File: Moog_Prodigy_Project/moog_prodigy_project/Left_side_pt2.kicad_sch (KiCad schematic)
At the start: 61 parts, among them Q1 CA3046, Q15 BC549, Q2 CA3046, Q4 CA3046, Q6 BC549, SW1 Switch_4x4, SW4 Switch_4x4, U2A1 OPA134, U2B3 OPA134, U5 NE5532, U6 LT1011CN8, U7 AD8066ARM, U8 NE5532

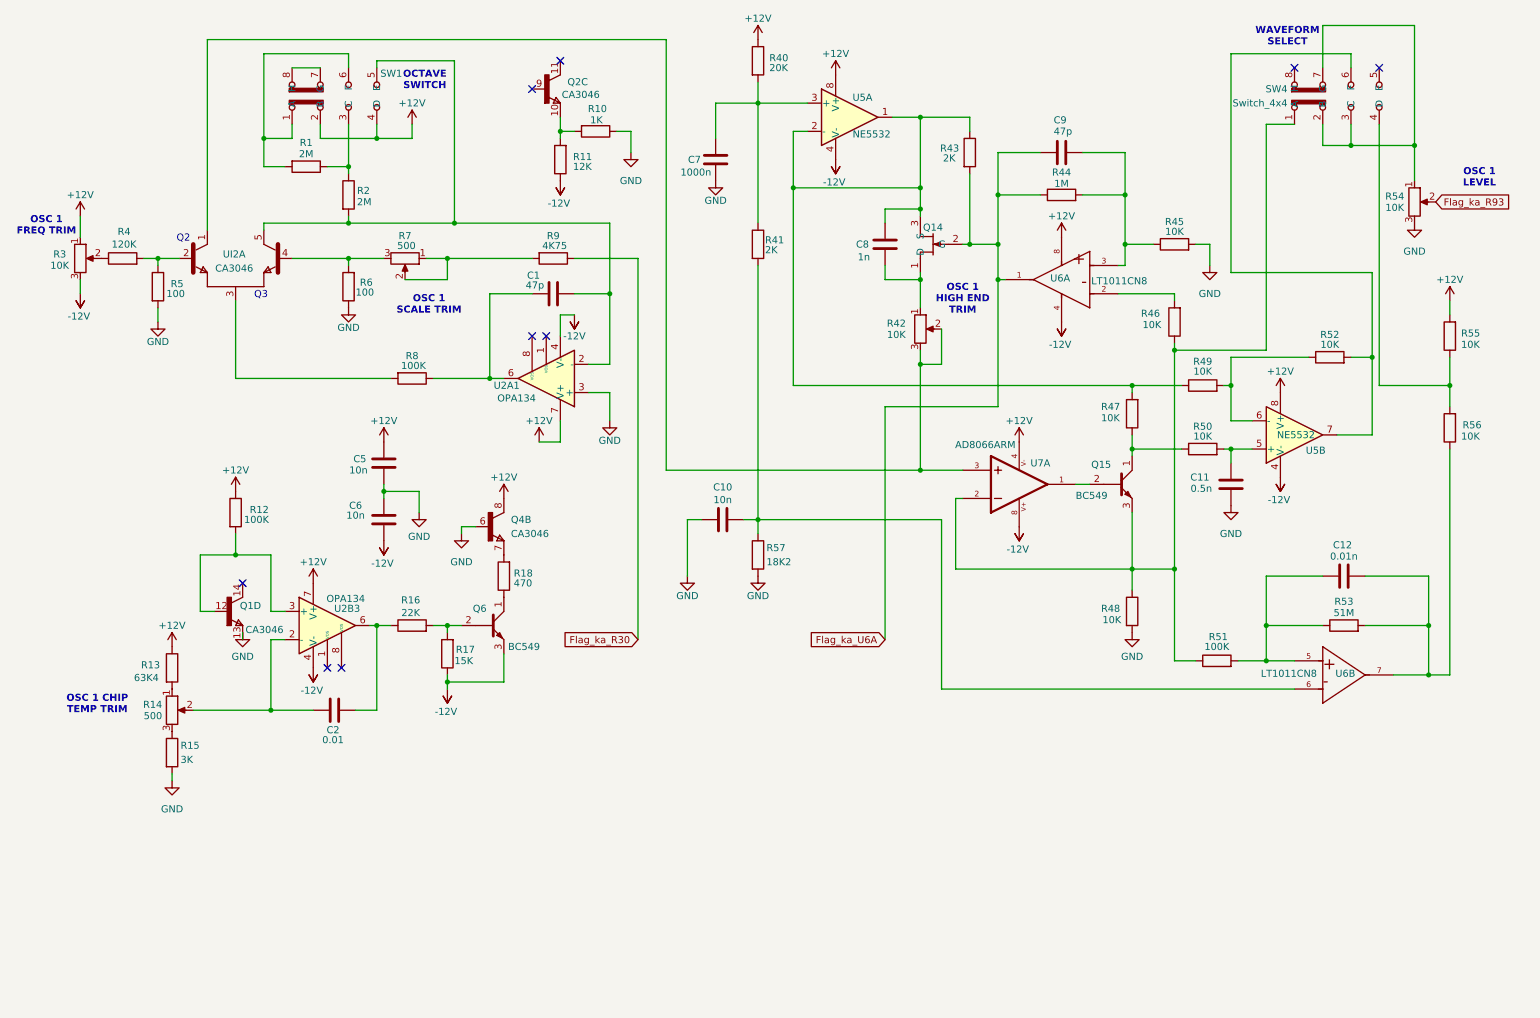
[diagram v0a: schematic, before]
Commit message: Spajanje projekta final 1
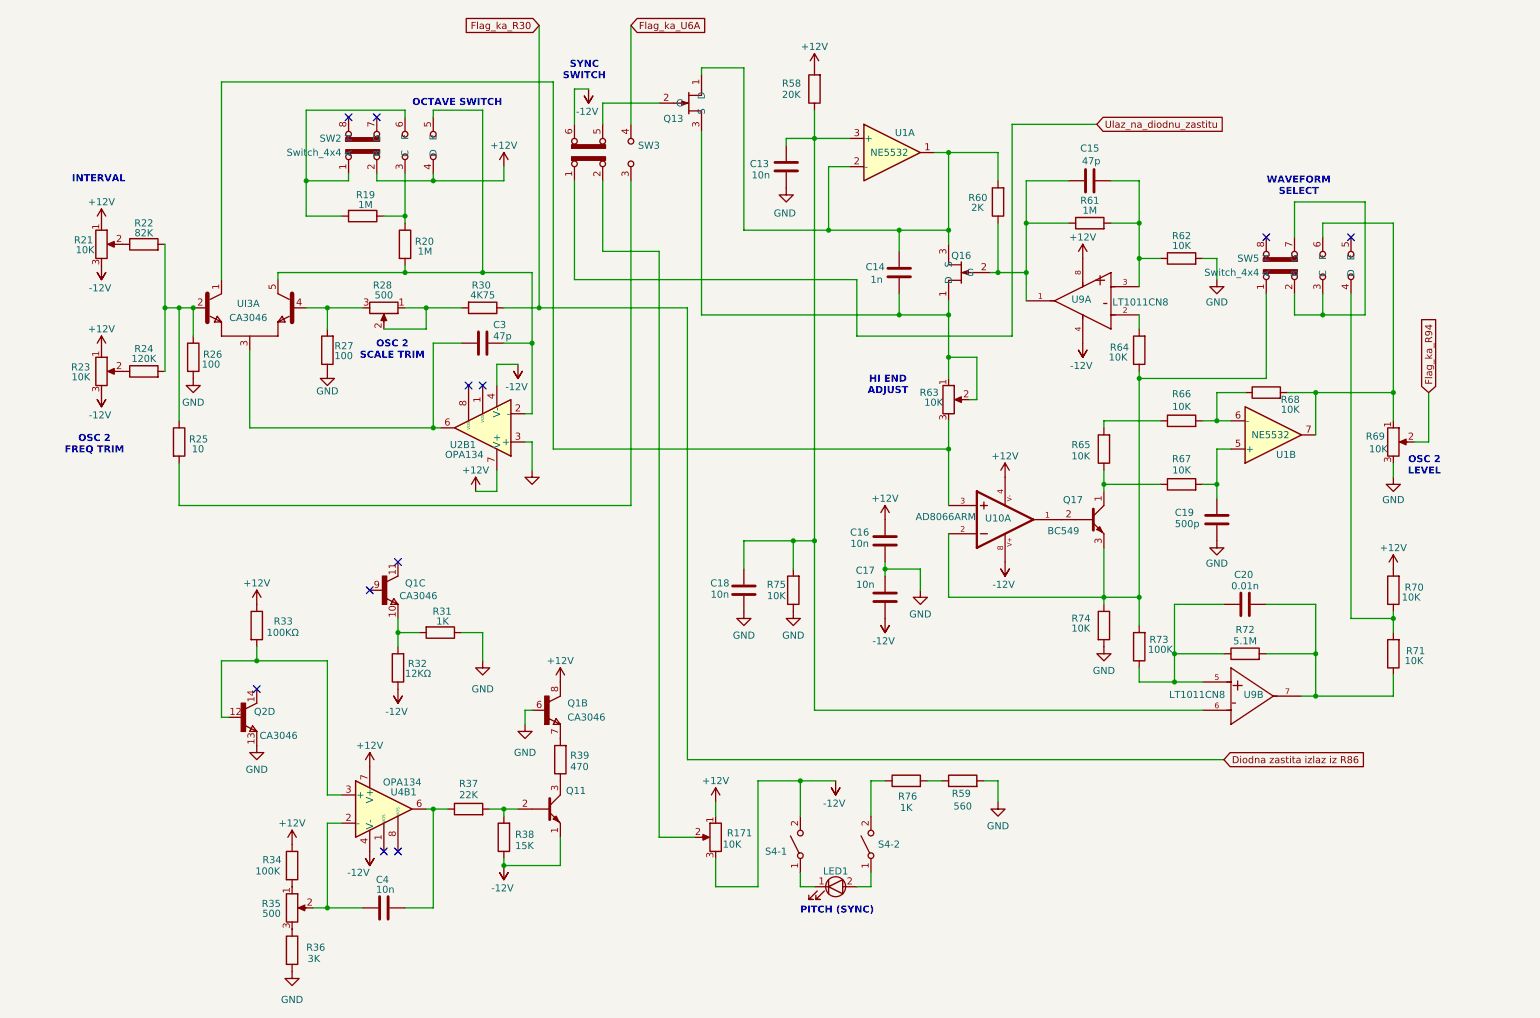
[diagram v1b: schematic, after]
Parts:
- removed C1, C9: 47p, Capacitor_THT:CP_Radial_D5.0mm_P2.50mm, symbol Device:C
- removed C10, C5, C6: 10n, Capacitor_THT:C_Disc_D3.8mm_W2.6mm_P2.50mm, symbol Device:C
- removed C11: 0.5n, Capacitor_THT:C_Disc_D3.8mm_W2.6mm_P2.50mm, symbol Device:C
- removed C12: 0.01n, Capacitor_THT:C_Disc_D3.8mm_W2.6mm_P2.50mm, symbol Device:C
- removed C2: 0.01, Capacitor_THT:C_Disc_D3.8mm_W2.6mm_P2.50mm, symbol Device:C
- removed C7: 1000n, Capacitor_THT:CP_Radial_D5.0mm_P2.50mm, symbol Device:C
- removed C8: 1n, Capacitor_THT:C_Disc_D3.8mm_W2.6mm_P2.50mm, symbol Device:C
- removed Q1, Q2, Q4, UI2: CA3046, CA3046:DIL14, symbol CA3046:CA3046
- removed Q14: ~, BF256C:TO92127P478H483-3, symbol Transistor_FET:BF256C
- removed Q15, Q6: BC549, Package_TO_SOT_THT:TO-92_Inline, symbol Transistor_BJT:BC549
- removed R1, R2: 2M, Resistor_THT:R_Axial_DIN0207_L6.3mm_D2.5mm_P7.62mm_Horizontal, symbol Device:R
- removed R10: 1K, Resistor_THT:R_Axial_DIN0207_L6.3mm_D2.5mm_P7.62mm_Horizontal, symbol Device:R
- removed R11: 12K, Resistor_THT:R_Axial_DIN0207_L6.3mm_D2.5mm_P7.62mm_Horizontal, symbol Device:R
- removed R12, R51, R8: 100K, Resistor_THT:R_Axial_DIN0207_L6.3mm_D2.5mm_P7.62mm_Horizontal, symbol Device:R
- removed R13: 63K4, Resistor_THT:R_Axial_DIN0207_L6.3mm_D2.5mm_P7.62mm_Horizontal, symbol Device:R
- removed R14, R7: 500, Resistor_THT:R_Axial_DIN0207_L6.3mm_D2.5mm_P7.62mm_Horizontal, symbol Device:R_Potentiometer
- removed R15: 3K, Resistor_THT:R_Axial_DIN0207_L6.3mm_D2.5mm_P7.62mm_Horizontal, symbol Device:R
- removed R16: 22K, Resistor_THT:R_Axial_DIN0207_L6.3mm_D2.5mm_P7.62mm_Horizontal, symbol Device:R
- removed R17: 15K, Resistor_THT:R_Axial_DIN0207_L6.3mm_D2.5mm_P7.62mm_Horizontal, symbol Device:R
- removed R18: 470, Resistor_THT:R_Axial_DIN0207_L6.3mm_D2.5mm_P7.62mm_Horizontal, symbol Device:R
- removed R3, R42, R54: 10K, Resistor_THT:R_Axial_DIN0207_L6.3mm_D2.5mm_P7.62mm_Horizontal, symbol Device:R_Potentiometer
- removed R4: 120K, Resistor_THT:R_Axial_DIN0207_L6.3mm_D2.5mm_P7.62mm_Horizontal, symbol Device:R
- removed R40: 20K, Resistor_THT:R_Axial_DIN0207_L6.3mm_D2.5mm_P7.62mm_Horizontal, symbol Device:R
- removed R41, R43: 2K, Resistor_THT:R_Axial_DIN0207_L6.3mm_D2.5mm_P7.62mm_Horizontal, symbol Device:R
- removed R44: 1M, Resistor_THT:R_Axial_DIN0207_L6.3mm_D2.5mm_P7.62mm_Horizontal, symbol Device:R
- removed R45, R46, R47, R48, R49, R50, R52, R55, R56: 10K, Resistor_THT:R_Axial_DIN0207_L6.3mm_D2.5mm_P7.62mm_Horizontal, symbol Device:R
- removed R5, R6: 100, Resistor_THT:R_Axial_DIN0207_L6.3mm_D2.5mm_P7.62mm_Horizontal, symbol Device:R
- removed R53: 51M, Resistor_THT:R_Axial_DIN0207_L6.3mm_D2.5mm_P7.62mm_Horizontal, symbol Device:R
- removed R57: 18K2, Resistor_THT:R_Axial_DIN0207_L6.3mm_D2.5mm_P7.62mm_Horizontal, symbol Device:R
- removed R9: 4K75, Resistor_THT:R_Axial_DIN0207_L6.3mm_D2.5mm_P7.62mm_Horizontal, symbol Device:R
- removed SW1, SW4: Switch_4x4, SLW-1575662-5A-S-D_Switch_4x4:SW_SLW-1575662-5A-S-D, symbol Power_supply:SW_Slide_DPDT_4x4
- removed U2A1, U2B3: OPA134, OPA134PA:DIP794W45P254L959H508Q8, symbol Amplifier_Operational:OPA134
- removed U5, U8: NE5532, NE5532AP:DIP794W45P254L1016H508Q8, symbol Amplifier_Operational:NE5532
- removed U6: LT1011CN8, Package_DIP:DIP-8_W7.62mm_Socket, symbol LM393BIPWR:LM393BIPWR
- removed U7: AD8066ARM, AD8066ARM:SOP65P490X110-8N, symbol AD8066ARM:AD8066ARM
- added C13, C16, C17, C18, C4: 10n, Capacitor_THT:C_Disc_D3.8mm_W2.6mm_P2.50mm, symbol Device:C
- added C14: 1n, Capacitor_THT:C_Disc_D3.8mm_W2.6mm_P2.50mm, symbol Device:C
- added C15, C3: 47p, Capacitor_THT:CP_Radial_D5.0mm_P2.50mm, symbol Device:C
- added C19: 500p, Capacitor_THT:CP_Radial_D5.0mm_P2.50mm, symbol Device:C
- added C20: 0.01n, Capacitor_THT:C_Disc_D3.8mm_W2.6mm_P2.50mm, symbol Device:C
- added LED1: ~, WP7113LGD:LED_WP7113LGD, symbol Device:LED_DIODA
- added Q1, Q2, UI3: CA3046, CA3046:DIL14, symbol CA3046:CA3046
- added Q11: BC107, Package_TO_SOT_THT:TO-18-3, symbol Transistor_BJT:BC107
- added Q13, Q16: ~, BF256C:TO92127P478H483-3, symbol Transistor_FET:BF256C
- added Q17: BC549, Package_TO_SOT_THT:TO-92_Inline, symbol Transistor_BJT:BC549
- added R171, R21, R23, R63, R69: 10K, Resistor_THT:R_Axial_DIN0207_L6.3mm_D2.5mm_P7.62mm_Horizontal, symbol Device:R_Potentiometer
- added R19, R20, R61: 1M, Resistor_THT:R_Axial_DIN0207_L6.3mm_D2.5mm_P7.62mm_Horizontal, symbol Device:R
- added R22: 82K, Resistor_THT:R_Axial_DIN0207_L6.3mm_D2.5mm_P7.62mm_Horizontal, symbol Device:R
- added R24: 120K, Resistor_THT:R_Axial_DIN0207_L6.3mm_D2.5mm_P7.62mm_Horizontal, symbol Device:R
- added R25: 10, Resistor_THT:R_Axial_DIN0207_L6.3mm_D2.5mm_P7.62mm_Horizontal, symbol Device:R
- added R26, R27: 100, Resistor_THT:R_Axial_DIN0207_L6.3mm_D2.5mm_P7.62mm_Horizontal, symbol Device:R
- added R28, R35: 500, Resistor_THT:R_Axial_DIN0207_L6.3mm_D2.5mm_P7.62mm_Horizontal, symbol Device:R_Potentiometer
- added R30: 4K75, Resistor_THT:R_Axial_DIN0207_L6.3mm_D2.5mm_P7.62mm_Horizontal, symbol Device:R
- added R31, R76: 1K, Resistor_THT:R_Axial_DIN0207_L6.3mm_D2.5mm_P7.62mm_Horizontal, symbol Device:R
- added R32: 12KΩ, Resistor_THT:R_Axial_DIN0207_L6.3mm_D2.5mm_P7.62mm_Horizontal, symbol Device:R
- added R33: 100KΩ, Resistor_THT:R_Axial_DIN0207_L6.3mm_D2.5mm_P7.62mm_Horizontal, symbol Device:R
- added R34, R73: 100K, Resistor_THT:R_Axial_DIN0207_L6.3mm_D2.5mm_P7.62mm_Horizontal, symbol Device:R
- added R36: 3K, Resistor_THT:R_Axial_DIN0207_L6.3mm_D2.5mm_P7.62mm_Horizontal, symbol Device:R
- added R37: 22K, Resistor_THT:R_Axial_DIN0207_L6.3mm_D2.5mm_P7.62mm_Horizontal, symbol Device:R
- added R38: 15K, Resistor_THT:R_Axial_DIN0207_L6.3mm_D2.5mm_P7.62mm_Horizontal, symbol Device:R
- added R39: 470, Resistor_THT:R_Axial_DIN0207_L6.3mm_D2.5mm_P7.62mm_Horizontal, symbol Device:R
- added R58: 20K, Resistor_THT:R_Axial_DIN0207_L6.3mm_D2.5mm_P7.62mm_Horizontal, symbol Device:R
- added R59: 560, Resistor_THT:R_Axial_DIN0207_L6.3mm_D2.5mm_P7.62mm_Horizontal, symbol Device:R
- added R60: 2K, Resistor_THT:R_Axial_DIN0207_L6.3mm_D2.5mm_P7.62mm_Horizontal, symbol Device:R
- added R62, R64, R65, R66, R67, R68, R70, R71, R74, R75: 10K, Resistor_THT:R_Axial_DIN0207_L6.3mm_D2.5mm_P7.62mm_Horizontal, symbol Device:R
- added R72: 5.1M, Resistor_THT:R_Axial_DIN0207_L6.3mm_D2.5mm_P7.62mm_Horizontal, symbol Device:R
- added S4-1, S4-2: SW_SPST, L101011ML04Q_1x1:SW_L101011ML04Q, symbol Switch:SW_SPST
- added SW2, SW5: Switch_4x4, SLW-1575662-5A-S-D_Switch_4x4:SW_SLW-1575662-5A-S-D, symbol Power_supply:SW_Slide_DPDT_4x4
- added SW3: SW_Slide_DPDT_3x3, CL-SB-22A-02T_3x3:SW_CL-SB-22A-02T, symbol Switch:SW_Slide_DPDT
- added U1: NE5532, NE5532AP:DIP794W45P254L1016H508Q8, symbol Amplifier_Operational:NE5532
- added U10: AD8066ARM, AD8066ARM:SOP65P490X110-8N, symbol AD8066ARM:AD8066ARM
- added U2B1, U4B1: OPA134, OPA134PA:DIP794W45P254L959H508Q8, symbol Amplifier_Operational:OPA134
- added U9: LT1011CN8, Package_DIP:DIP-8_W7.62mm_Socket, symbol LM393BIPWR:LM393BIPWR
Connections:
- net +12V: now also C16.2, Q1.8, R171.1, R21.1, R23.1, R33.1, R34.1, R58.2, R70.2, SW2.2 (B), SW2.4 (D), U10.4, U2B1.7 (V+), U4B1.7 (V+), U9.8
- net -12V: now also C17.1, Q11.1 (E), R171.3, R21.3, R23.3, R32.1, R38.1, S4-1.2 (B), SW3.6 (C), U10.8, U2B1.4 (V-), U4B1.4 (V-), U9.4
- net Flag_ka_U6A: now also SW3.4 (A)
- net GND: now also C13.1, C16.1, C17.2, C18.1, C19.1, Q1.6, Q2.13, R26.2, R27.1, R31.1, R36.2, R59.2, R62.2, R69.3, R74.2, R75.1, U2B1.3 (+)
- new net: Q2.12, R33.2, U4B1.3 (+)
- new net: R21.2, R22.1
- new net: R22.2, R24.2, R25.1, R26.1, UI3.2
- new net: R59.1, R76.2
- new net: C15.1, Q16.2 (G), R60.1, R61.1, U9.1
- new net: C15.2, R61.2, R62.1, U9.3
- new net: Q17.3 (E), R64.1, R73.2, R74.1, SW5.1 (A), U10.2
- new net: R64.2, U9.2
- new net: R28.1, R28.2, R30.2
- new net: R27.2, R28.3, UI3.4
- new net: C14.1, Q13.3 (S), Q16.1 (D), R63.1, R63.2
- new net: C14.2, Q13.1 (D), Q16.3 (S), R60.2, U1.1, U1.2 (-)
- new net: C13.2, C18.2, R58.1, R75.2, U1.3 (+), U9.6
- new net: Q13.2 (G), SW3.5 (B)
- new net: Q17.1 (C), R65.1, R67.1
- new net: C19.2, R67.2, U1.5 (+)
- new net: R66.2, R68.1, U1.6 (-)
- new net: R68.2, R69.1, SW5.6 (F), U1.7
- new net: LED1.1, S4-1.1 (A)
- new net: C4.2, R37.1, U4B1.6
- new net: Q11.2 (B), R37.2, R38.2
- new net: R25.2, SW3.3 (C)
- new net: Q1.10, R31.2, R32.2
- new net: R63.3, U10.3, UI3.1
- new net: C3.1, U2B1.6, UI3.3
- new net: C3.2, R20.2, SW2.5 (E), U2B1.2 (-), UI3.5
- new net: C4.1, R35.2, U4B1.2 (-)
- new net: R65.2, R66.1
- new net: R35.3, R36.1
- new net: LED1.2, S4-2.1 (A)
- new net: R76.1, S4-2.2 (B)
- new net: C20.1, R71.1, R72.2, U9.7
- new net: R70.1, R71.2, SW5.4 (D)
- new net: R34.2, R35.1
- new net: R19.1, R20.1, SW2.3 (C)
- new net: Q17.2 (B), U10.1
- new net: R19.2, SW2.1 (A), SW2.6 (F)
- new net: R171.2, SW3.2 (B)
- new net: Q11.3 (C), R39.1
- new net: Q1.7, R39.2
- new net: R23.2, R24.1
- new net: C20.2, R72.1, R73.1, U9.5
- new net: SW5.2 (B), SW5.3 (C), SW5.7 (G)
- new net Diodna zastita izlaz iz R86: R30.1
- new net Flag_ka_R94: R69.2
- new net Ulaz_na_diodnu_zastitu: SW3.1 (A)
- no-connect marks 9 -> 11
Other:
- note added: "HI END ADJUST"
- note added: "INTERVAL"
- note added: "OSC 2 FREQ TRIM"
- note added: "OSC 2 LEVEL"
- note added: "OSC 2 SCALE TRIM"
- note added: "PITCH (SYNC)"
- note added: "SYNC SWITCH"
- note removed: "OSC 1 CHIP TEMP TRIM"
- note removed: "OSC 1 FREQ TRIM"
- note removed: "OSC 1 HIGH END TRIM"
- note removed: "OSC 1 LEVEL"
- note removed: "OSC 1 SCALE TRIM"
- note removed: "Q2"
- note removed: "Q3"
